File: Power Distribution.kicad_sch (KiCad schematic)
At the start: 16 parts, among them J1 Conn_01x02, J2 Conn_01x02, J3 Conn_01x02, J4 Conn_01x02, Q1 Q_PMOS_DGS

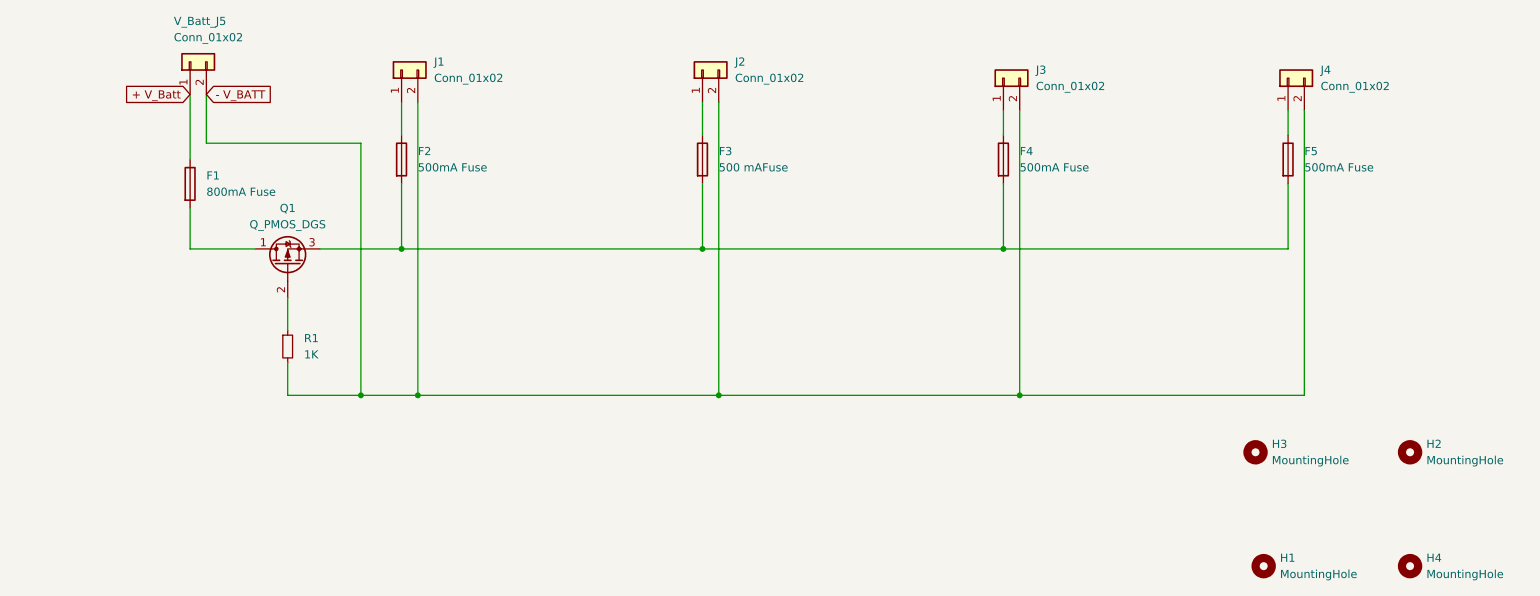
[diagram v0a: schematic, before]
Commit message: Add files via upload
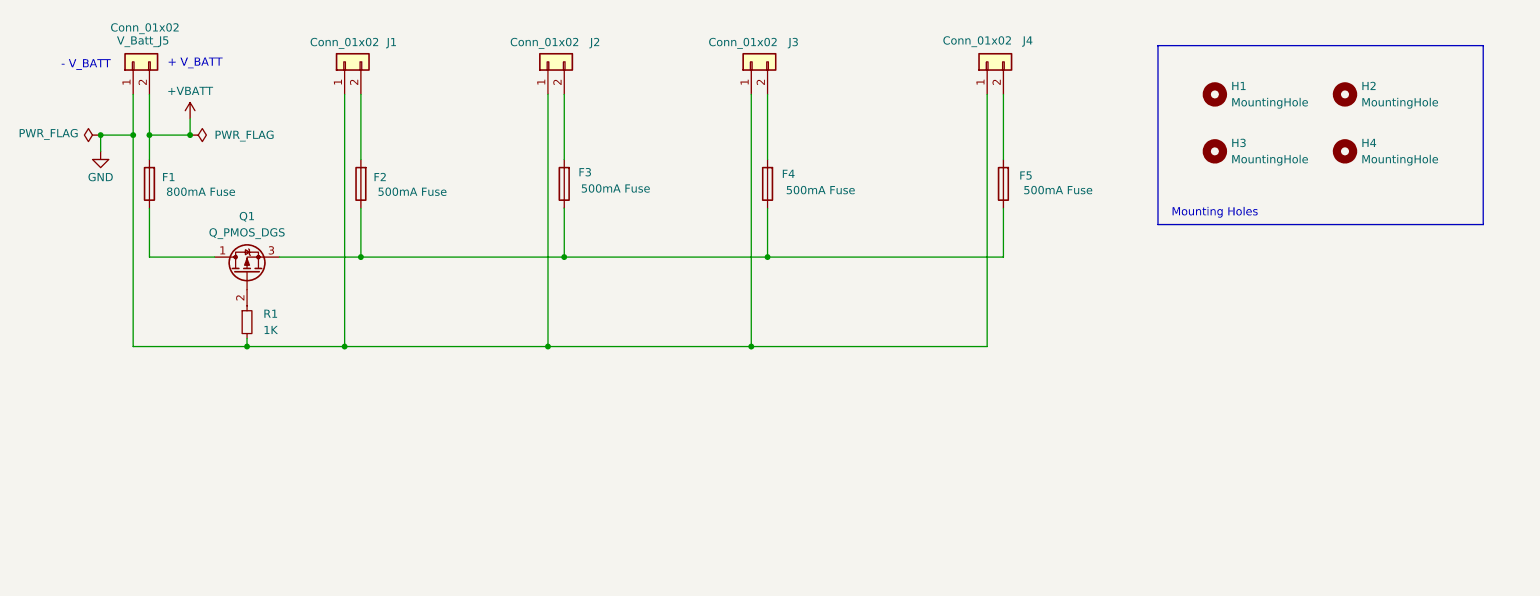
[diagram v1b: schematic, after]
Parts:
- F1, F2, F4, F5: footprint Fuse:Fuse_0603_1608Metric -> Fuse:Fuse_0805_2012Metric
- F3: value 500 mAFuse -> 500mA Fuse; footprint Fuse:Fuse_0603_1608Metric -> Fuse:Fuse_0805_2012Metric
- Q1: footprint Transistor_Packages:SOT23_Standard -> DMP3056L-7 2:SOT91P240X110-3N
- R1: footprint Resistor_SMD:R_0402_1005Metric -> Resistor_SMD:R_0805_2012Metric
- V_Batt_J5: value Conn_01x02 -> Conn_01x02
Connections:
- net at F4.1: now also F2.1, F3.1, F5.1, Q1.3 (S); no longer J3.1 (Pin_1)
- net GND: now reaches J2.1 (Pin_1)
- net GND: now also J1.1 (Pin_1), J3.1 (Pin_1), J4.1 (Pin_1), R1.2, V_Batt_J5.1 (Pin_1); no longer F3.1
- net at Q1.1 (D): now also F1.1; no longer F1.2
- removed net + V_Batt: F1.1, V_Batt_J5.1 (Pin_1)
- removed net - V_BATT: J1.2 (Pin_2), J2.2 (Pin_2), J3.2 (Pin_2), J4.2 (Pin_2), R1.2, V_Batt_J5.2 (Pin_2)
- new net: F4.2, J3.2 (Pin_2)
- new net: F3.2, J2.2 (Pin_2)
- new net: F5.2, J4.2 (Pin_2)
- new net: F2.2, J1.2 (Pin_2)
- new net +VBATT: F1.2, V_Batt_J5.2 (Pin_2)
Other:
- note added: "+ V_BATT"
- note added: "- V_BATT"
- note added: "Mounting Holes"
- moved on the sheet: F1, F2, F3, F5, H1, H2, H3, H4, J1, J2, J3, Q1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
